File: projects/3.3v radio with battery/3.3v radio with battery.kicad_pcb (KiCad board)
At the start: 2 copper layers, 130 x 80 mm, 17 parts, among them J1 USB_B

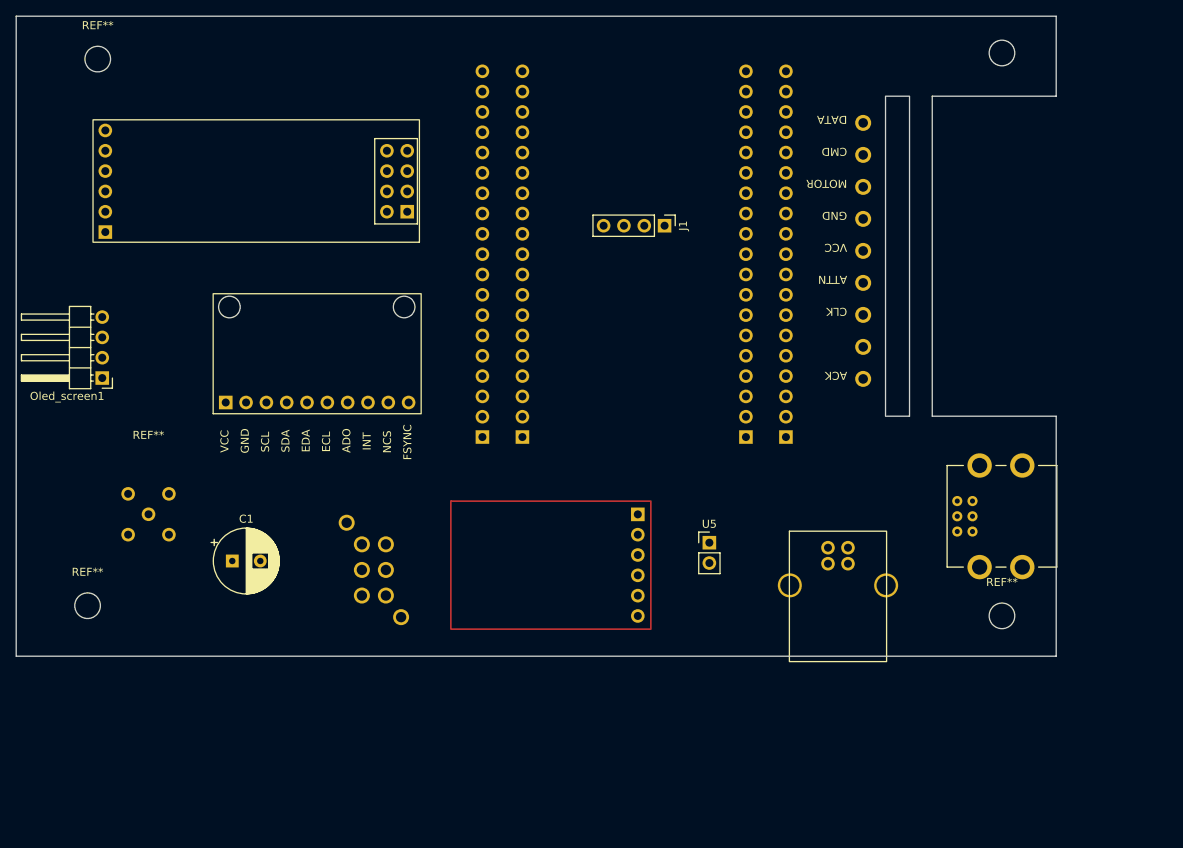
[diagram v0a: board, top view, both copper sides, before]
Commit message: a lot of project updates
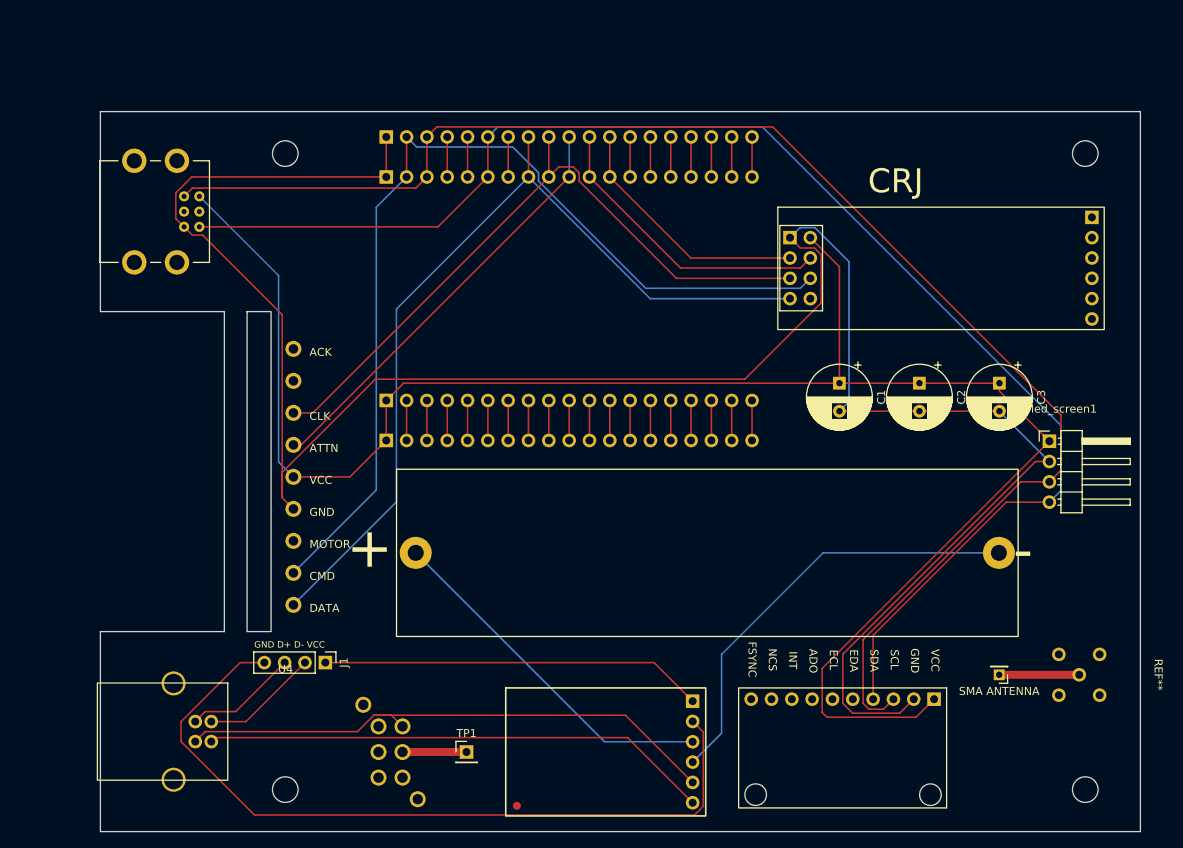
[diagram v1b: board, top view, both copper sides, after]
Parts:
- removed the REF** at (211.8, 41.4)
- removed the REF** at (211.8, 111.8)
- removed the REF** at (133.2, 93.3)
- removed the REF** at (98.8, 42.2)
- removed the REF** at (97.5, 110.5)
- added C2: CP_Axial_L10.0mm_D4.5mm_P15.00mm, Capacitor_THT:CP_Radial_D8.0mm_P3.50mm, F.Cu at (201.5, 82.7)
- added C3: CP_Axial_L10.0mm_D4.5mm_P15.00mm, Capacitor_THT:CP_Radial_D8.0mm_P3.50mm, F.Cu at (211.5, 82.7)
- added REF**: MountingHole_3.2mm_M3, MountingHole:MountingHole_3.2mm_M3, F.Cu at (222.2, 54.0)
- added REF**: MountingHole_3.2mm_M3, MountingHole:MountingHole_3.2mm_M3, F.Cu at (222.2, 133.5)
- added REF**: MountingHole_3.2mm_M3, MountingHole:MountingHole_3.2mm_M3, F.Cu at (122.2, 54.0)
- added REF**: MountingHole_3.2mm_M3, MountingHole:MountingHole_3.2mm_M3, F.Cu at (122.2, 133.5)
- added SMA ANTENNA: PinHeader_1x01_P2.00mm_Vertical, Connector_PinHeader_2.00mm:PinHeader_1x01_P2.00mm_Vertical, F.Cu at (211.5, 119.1)
- added TP1: TestPoint, Connector_PinHeader_2.54mm:PinHeader_1x01_P2.54mm_Vertical, F.Cu at (144.9, 128.8)
- added U6: ~, Footprints_cez:Switch A03 PS-22F03, F.Cu at (135.3, 116.1)
- U5: footprint Connector_PinHeader_2.54mm:PinHeader_1x02_P2.54mm_Vertical -> Footprints_cez:BH-18650-PC2
- moved REF** 129.1 mm to (230.9, 119.1), turned to -90 degrees
- moved Oled_screen1 118.7 mm to (217.8, 89.9), turned to 0 degrees
- moved U1 112.6 mm to (105.9, 61.2), turned to 90 degrees
- moved MPU1 111.5 mm to (209.5, 127.4), turned to -90 degrees
- moved C1 79.1 mm to (191.5, 82.7), turned to -90 degrees
- moved U4 75.1 mm to (124.3, 126.1), turned to -90 degrees
- moved J1 69.1 mm to (127.3, 117.6)
- moved U2 66.0 mm to (127.7, 91.1), turned to 0 degrees
- moved NRF1 48.0 mm to (185.3, 64.5), turned to 0 degrees
- moved U5 31.1 mm to (144.9, 96.1)
- moved U3 24.3 mm to (161.7, 114.3)
- moved ESP32-WROOM-32U1 20.7 mm to (147.1, 72.1), turned to 90 degrees
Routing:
- net Net-(MPU1-GND): track 0.00 -> 278.3 mm
- net Net-(ESP32-WROOM-32U1-3.3v): track 0.00 -> 226.3 mm
- net Net-(ESP32-WROOM-32U1-SCL/22): track 0.00 -> 184.0 mm
- net Net-(ESP32-WROOM-32U1-SDA/21): track 0.00 -> 178.3 mm
- net Net-(ESP32-WROOM-32U1-MOSI/23): track 0.00 -> 119.8 mm
- net Net-(ESP32-WROOM-32U1-MISO/19): track 0.00 -> 109.7 mm
- net Net-(J1-GND): track 0.00 -> 96.6 mm
- net Net-(ESP32-WROOM-32U1-SCK/18): track 0.00 -> 86.2 mm
- net Net-(U3-GND_IN): track 0.00 -> 71.2 mm
- net Net-(U3-VIN): track 0.00 -> 63.8 mm
- net Net-(U3-BAT_GND): track 0.00 -> 54.9 mm
- net Net-(ESP32-WROOM-32U1-SS/5): track 0.00 -> 53.3 mm
- net Net-(J1-VBUS): track 0.00 -> 47.9 mm
- net Net-(U3-BAT_POSITIVE): track 0.00 -> 44.4 mm
- net Net-(ESP32-WROOM-32U1-17): track 0.00 -> 37.8 mm
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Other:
- board size 130 x 80 mm -> 130 x 90 mm
- board text added: "CRJ"
- board text added: "GND D+ D- VCC"
